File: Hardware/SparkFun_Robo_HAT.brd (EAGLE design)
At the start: 65 x 56.5 mm, 237 parts, among them J11 EXT MTR PWR, J18 ISP, J2 RASPBERRYPI-40-PIN-GPIO_PTH_N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, J20 USB C, J23 CORTEX_JTAG_DEBUG_PTH, J7 EXT SERVO PWR, J8 EXT 5V PWR, Q1 310mA/60V/1.6Ω, Q23 20V/0.2A/8MHz/1.2Ω/1Vth, Q24 20V/0.2A/8MHz/1.2Ω/1Vth, Q27 20V/0.2A/8MHz/1.2Ω/1Vth, Q28 20V/0.2A/8MHz/1.2Ω/1Vth, Q4 310mA/60V/1.6Ω, Q5 20V/4.2A/52mΩ/1.4W, Q7 20V/4.2A/52mΩ/1.4W, Q9 20V/4.2A/52mΩ/1.4W, U1 PCA9685, U4 ATTINY84-ARDUINO, U5 DRV8835, U6 CY8C4245LQI-483, U7 9DoF IMU, U8 1.8V/100mA

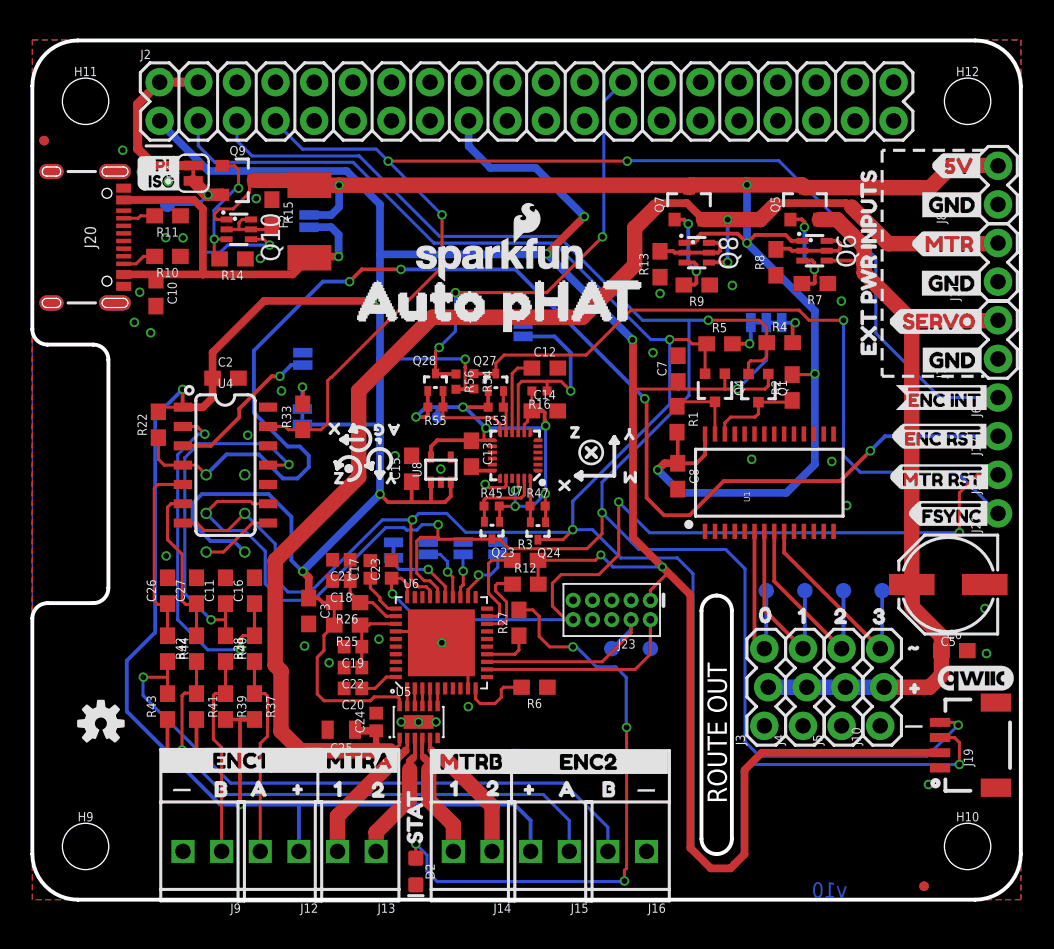
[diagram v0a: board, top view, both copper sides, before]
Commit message: moving to SMD stackable solution... 99 done
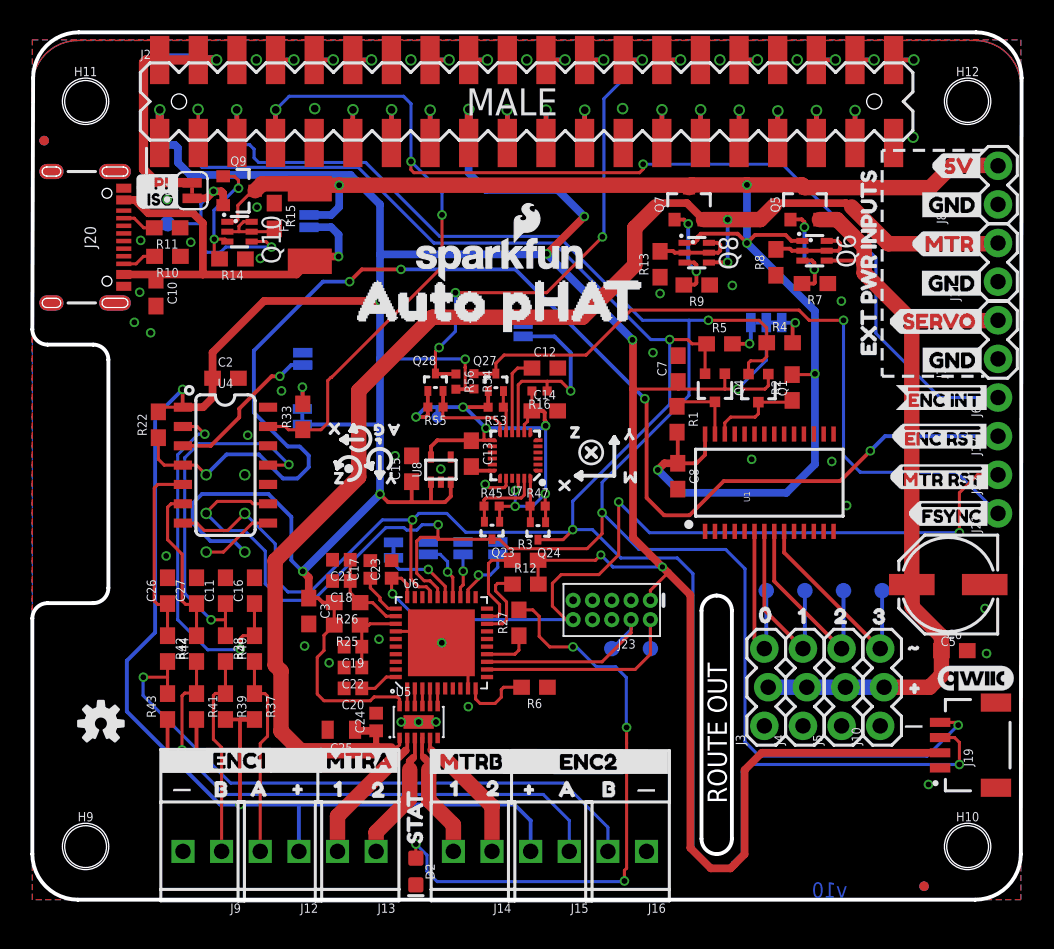
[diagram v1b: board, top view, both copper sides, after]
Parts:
- J19: value (none) -> QWIIC_RIGHT_ANGLE; device SparkFun-Connectors:1X04_1MM_RA -> SparkFun-Connectors:JST04_1MM_RA
- J2: value RASPBERRYPI-40-PIN-GPIO_PTH_NO_SHROUD -> RASPBERRYPI-40-PIN-GPIO_SMD_STACKABLE; device SparkFun-Connectors:2X20 -> SparkFun-Connectors:RASPBERRY_PI_HAT_40_PIN_SMD_STACKABLE
- TP0, TP1, TP2, TP3, TP7, TP8: value (none) -> TEST-POINT3X4
- TP4, TP5: value (none) -> TEST-POINTTP_15TH_THRU
- TP9: value (none) -> TEST-POINT3
- moved TP6 1.27 mm to (8.89, 44.5)
- moved U$32 1.20 mm to (6.86, 46.1)
- moved U$35 1.20 mm to (7.32, 47.1)
- moved JP4 1.15 mm to (10.5, 46.6)
- moved R11 0.79 mm to (8.86, 44.2)
- moved Q9 0.69 mm to (13.5, 46.6)
- moved R15 0.27 mm to (15.9, 45.0)
- moved F2 0.23 mm to (18.2, 44.4)
- moved Q10 0.16 mm to (13.6, 43.9)
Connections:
- new net CE0: J2.24, J2.24B
- new net GP12: J2.32, J2.32B
- new net GP13: J2.33, J2.33B
- new net GP16: J2.36, J2.36B
- new net GP17: J2.11, J2.11B
- new net GP18: J2.12, J2.12B
- new net GP19: J2.35, J2.35B
- new net GP20: J2.38, J2.38B
- new net GP21: J2.40, J2.40B
- new net GP22: J2.15, J2.15B
- new net GP23: J2.16, J2.16B
- new net GP24: J2.18, J2.18B
- new net GP25: J2.22, J2.22B
- new net GP26: J2.37, J2.37B
- new net GP27: J2.13, J2.13B
- new net GP5: J2.29, J2.29B
- new net GP6: J2.31, J2.31B
- new net ID_SC: J2.28, J2.28B
- new net ID_SD: J2.27, J2.27B
- new net PI_MISO: J2.21, J2.21B
- new net PI_MOSI: J2.19, J2.19B
- new net PI_RXI: J2.10, J2.10B
- new net PI_TXO: J2.8, J2.8B
- new net SCLK: J2.23, J2.23B
- net !ENC_INT: now also J2.7B
- net 3.3V: now also J2.17B, J2.1B
- net GND: now also J2.14B, J2.20B, J2.25B, J2.30B, J2.34B, J2.39B, J2.6B, J2.9B
- net IMU_INT_3.3V: now also J2.26B
- net N$20: now also J2.2B, J2.4B
- net SCL_3.3V: now also J2.5B
- net SDA_3.3V: now also J2.3B
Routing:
- net 3.3V: track 313.7 -> 322.1 mm, vias 13 -> 15
- net !ENC_INT: track 84.1 -> 92.1 mm, vias 3 -> 4
- net N$20: track 11.6 -> 19.3 mm, vias 0 -> 1
- net PI_MOSI: track 0.00 -> 4.51 mm, vias 0 -> 1
- net GP27: track 0.00 -> 4.51 mm, vias 0 -> 1
- net GP17: track 0.00 -> 4.51 mm, vias 0 -> 1
- net ID_SD: track 0.00 -> 4.51 mm, vias 0 -> 1
- net GP5: track 0.00 -> 4.51 mm, vias 0 -> 1
- net SCLK: track 0.00 -> 4.46 mm, vias 0 -> 1
- net PI_MISO: track 0.00 -> 4.46 mm, vias 0 -> 1
- net GP6: track 0.00 -> 4.46 mm, vias 0 -> 1
- net GP22: track 0.00 -> 4.46 mm, vias 0 -> 1
- net GP26: track 0.00 -> 4.41 mm, vias 0 -> 1
- net GP19: track 0.00 -> 4.41 mm, vias 0 -> 1
- net GP13: track 0.00 -> 4.36 mm, vias 0 -> 1
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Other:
- board size 65 x 56.5 mm -> 65.1 x 57 mm
